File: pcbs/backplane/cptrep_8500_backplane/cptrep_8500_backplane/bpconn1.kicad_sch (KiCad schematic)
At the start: 1 part, among them J1 cpt-backplane_100

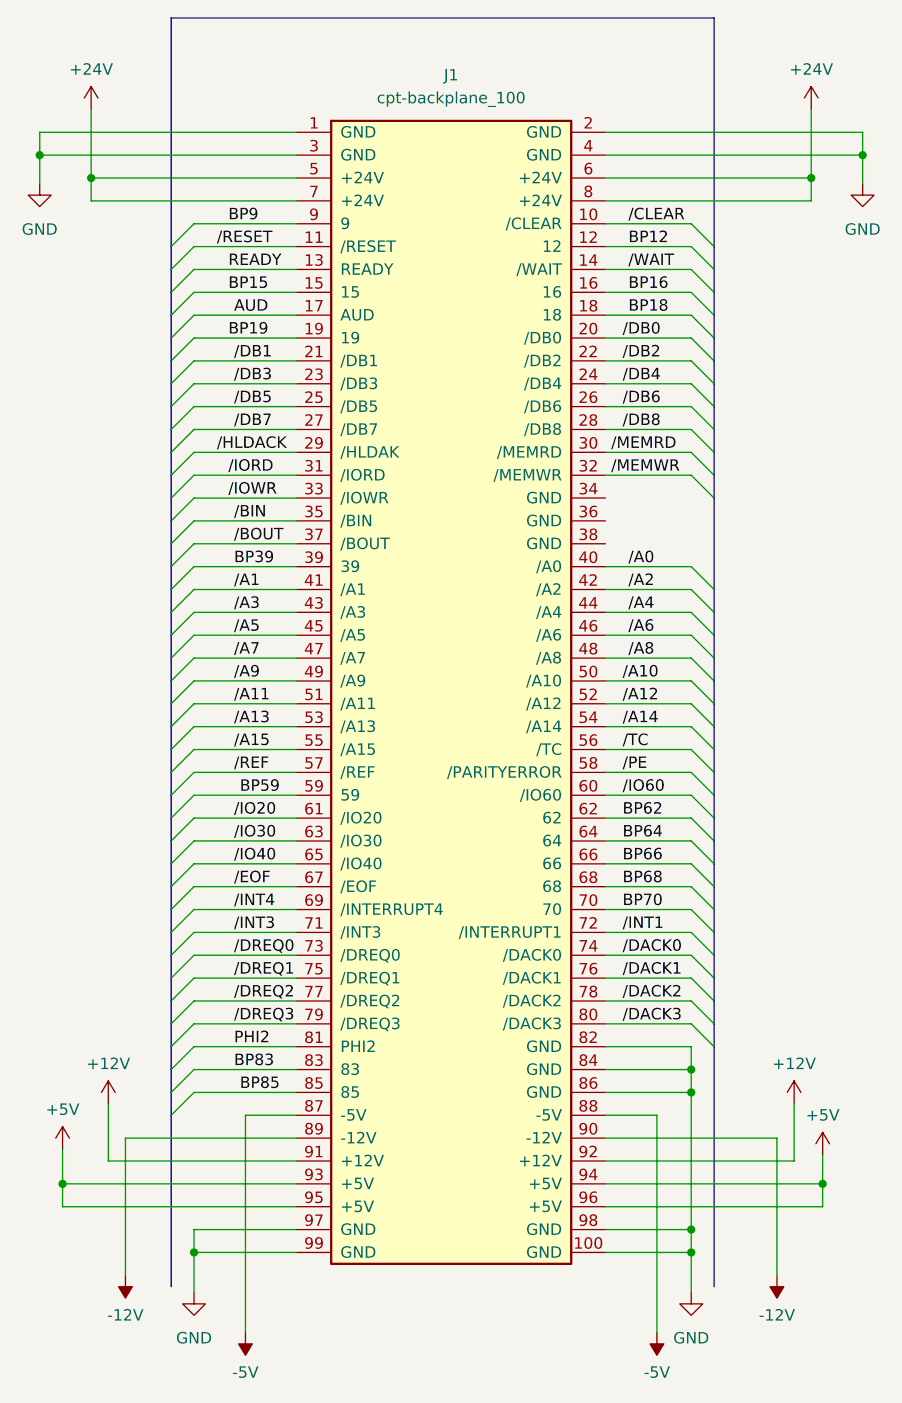
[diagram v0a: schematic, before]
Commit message: "Update"
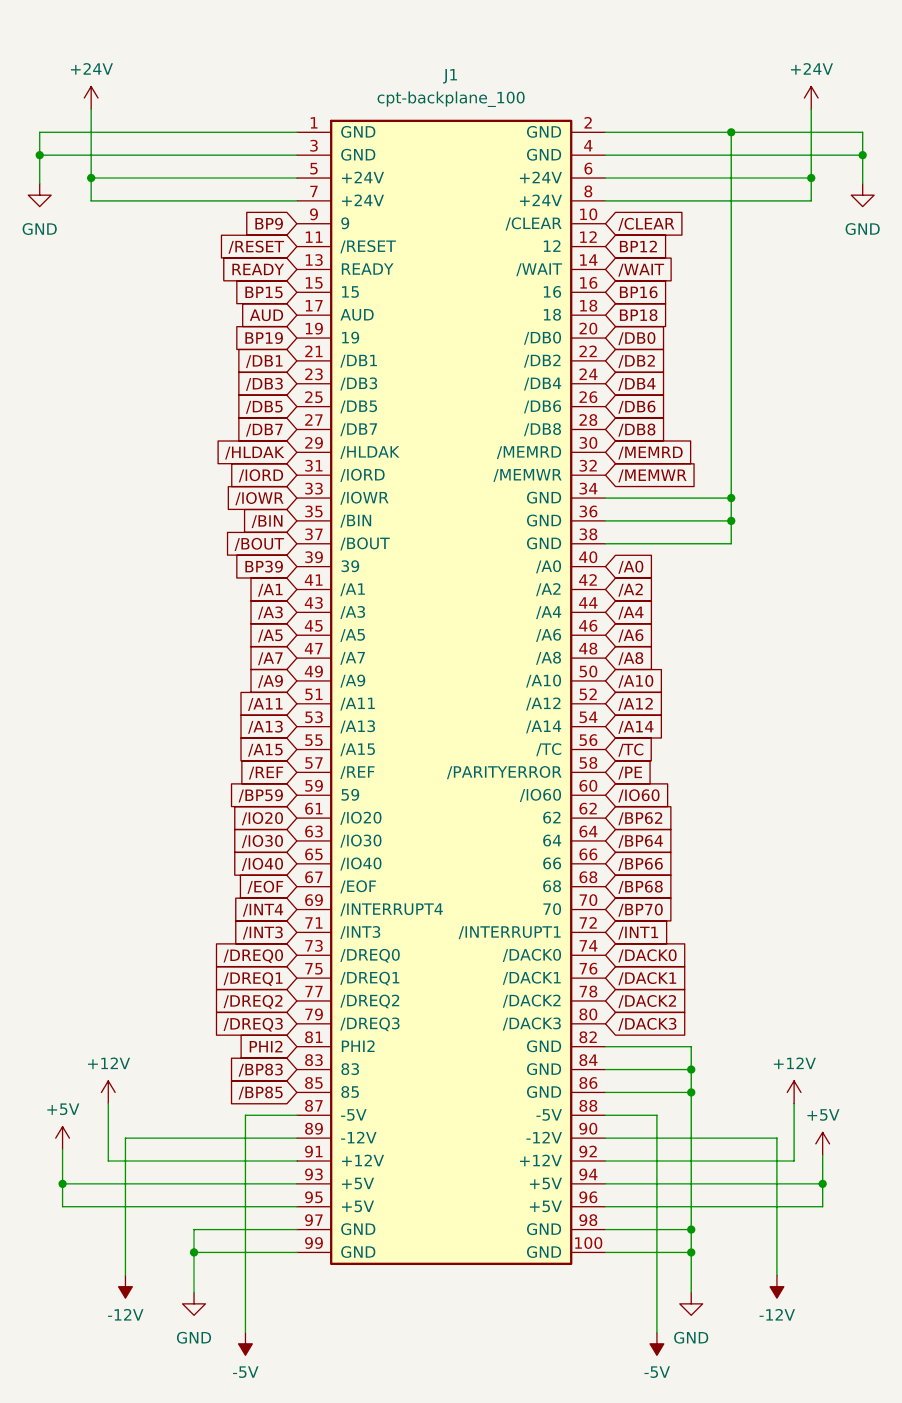
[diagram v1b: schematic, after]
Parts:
- J1: footprint (none) -> ajm-cpt:cpt-8500-backplane-connector
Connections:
- net GND: now also J1.34 (GND), J1.36 (GND), J1.38 (GND)
- net /BP68: now reaches J1.68
- net BP59 renamed /BP59
- net BP62 renamed /BP62
- net BP64 renamed /BP64
- net BP66 renamed /BP66
- net BP70 renamed /BP70
- net BP83 renamed /BP83
- net BP85 renamed /BP85
- net /HLDACK renamed /HLDAK
